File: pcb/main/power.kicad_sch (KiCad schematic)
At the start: 6 parts

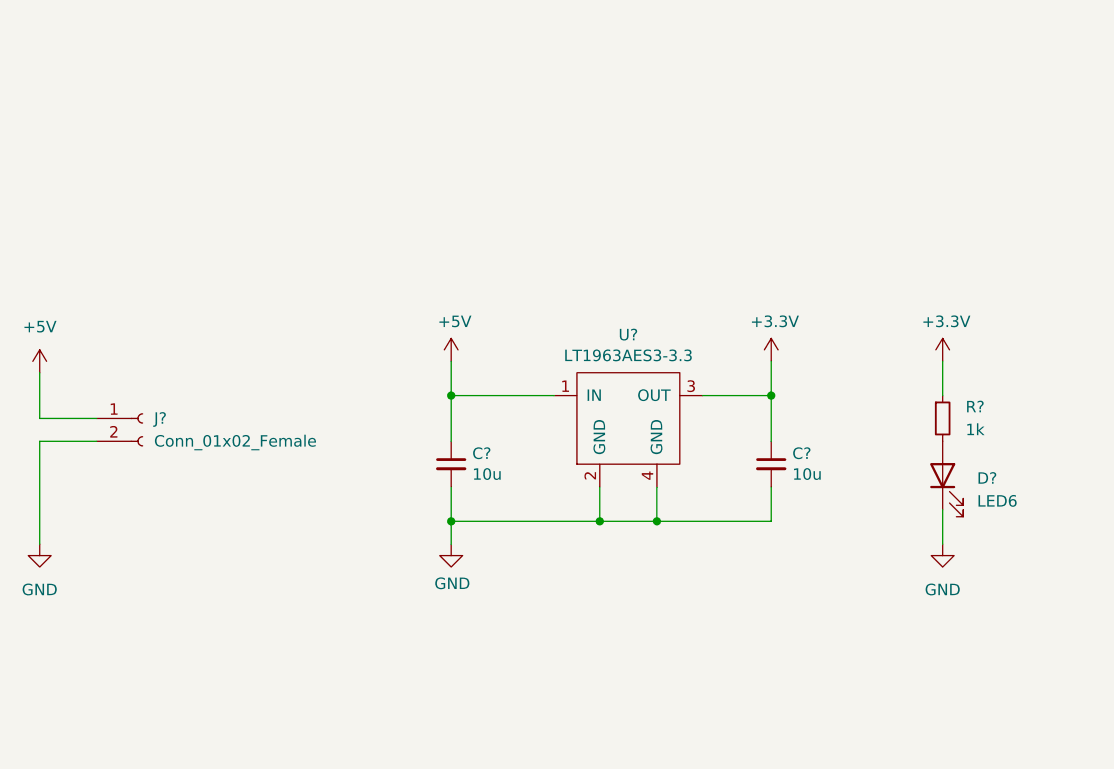
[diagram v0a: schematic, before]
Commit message: chore: add circuit git changes
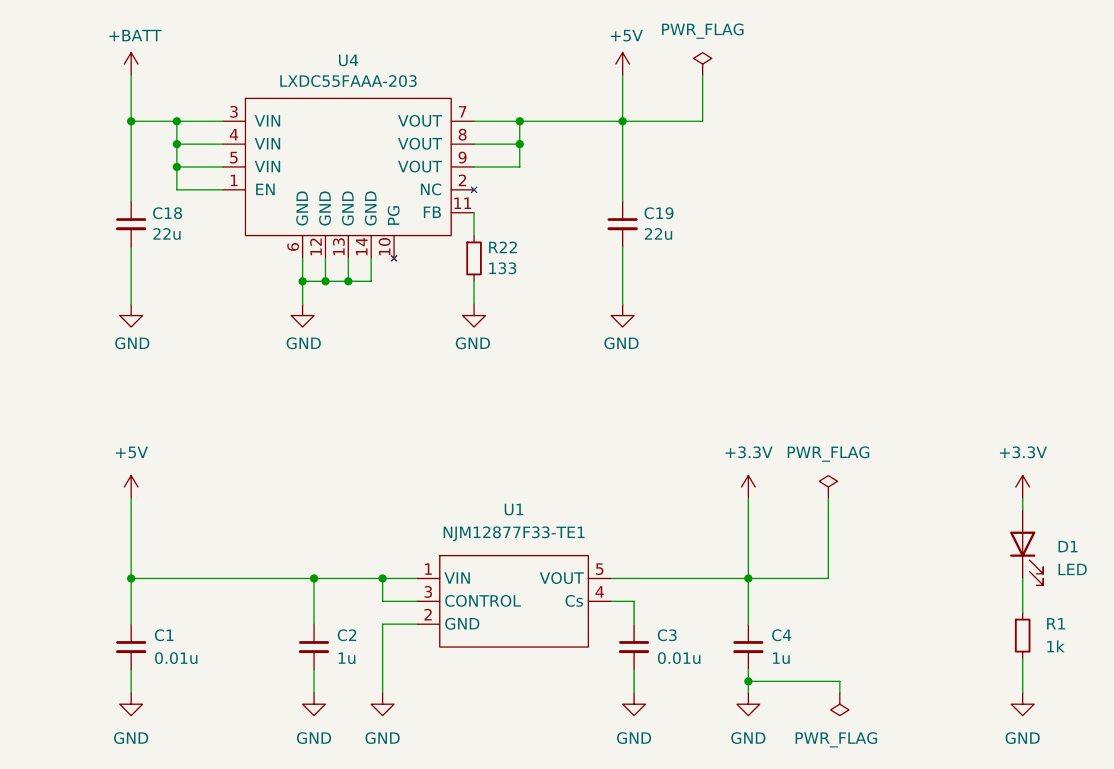
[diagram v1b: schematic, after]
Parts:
- removed C? (x2): 10u, Capacitor_SMD:C_0603_1608Metric_Pad1.08x0.95mm_HandSolder, symbol Device:C_Small
- removed D?: LED6, LED_SMD:LED_0402_1005Metric, symbol Device:LED
- removed J?: Conn_01x02_Female, symbol Connector:Conn_01x02_Female
- removed R?: 1k, Resistor_SMD:R_0201_0603Metric, symbol Device:R_Small
- removed U?: LT1963AES3-3.3, Package_TO_SOT_SMD:SOT-223, symbol My_Device:LT1963AES3-3.3
- added C1, C3: 0.01u, Capacitor_SMD:C_0603_1608Metric_Pad1.08x0.95mm_HandSolder, symbol Device:C_Small
- added C18, C19: 22u, Capacitor_SMD:C_0603_1608Metric_Pad1.08x0.95mm_HandSolder, symbol Device:C_Small
- added C2, C4: 1u, Capacitor_SMD:C_0603_1608Metric_Pad1.08x0.95mm_HandSolder, symbol Device:C_Small
- added D1: LED, LED_SMD:LED_0402_1005Metric, symbol Device:LED
- added R1: 1k, Resistor_SMD:R_0603_1608Metric_Pad0.98x0.95mm_HandSolder, symbol Device:R_Small
- added R22: 133, Resistor_SMD:R_0603_1608Metric_Pad0.98x0.95mm_HandSolder, symbol Device:R_Small
- added U1: NJM12877F33-TE1, Package_TO_SOT_SMD:SOT-23-5_HandSoldering, symbol bldc_lib:NJM12877F33-TE1
- added U4: LXDC55FAAA-203, cubli:LXDC55FAAA-203, symbol My_Device:LXDC55FAAA-203
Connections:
- net +3.3V: now also C4.1, D1.2 (A), U1.5 (VOUT)
- net +5V: now also C1.1, C19.1, C2.1, U1.1 (VIN), U1.3 (CONTROL), U4.7 (VOUT), U4.8 (VOUT), U4.9 (VOUT)
- net GND: now also C1.2, C18.2, C19.2, C2.2, C3.2, C4.2, R1.2, R22.2, U1.2 (GND), U4.12 (GND), U4.13 (GND), U4.14 (GND), U4.6 (GND)
- new net: R22.1, U4.11 (FB)
- new net: C3.1, U1.4 (Cs)
- new net: D1.1 (K), R1.1
- new net +BATT: C18.1, U4.1 (EN), U4.3 (VIN), U4.4 (VIN), U4.5 (VIN)
